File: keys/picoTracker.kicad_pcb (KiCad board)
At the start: 2 copper layers, 75 x 64.5 mm, 15 parts, among them J1 Conn_01x10, SW1 LEFT, SW2 DOWN, SW3 RIGHT, SW4 UP, SW5 LT, SW6 B, SW7 A, SW8 RT, SW9 PLAY

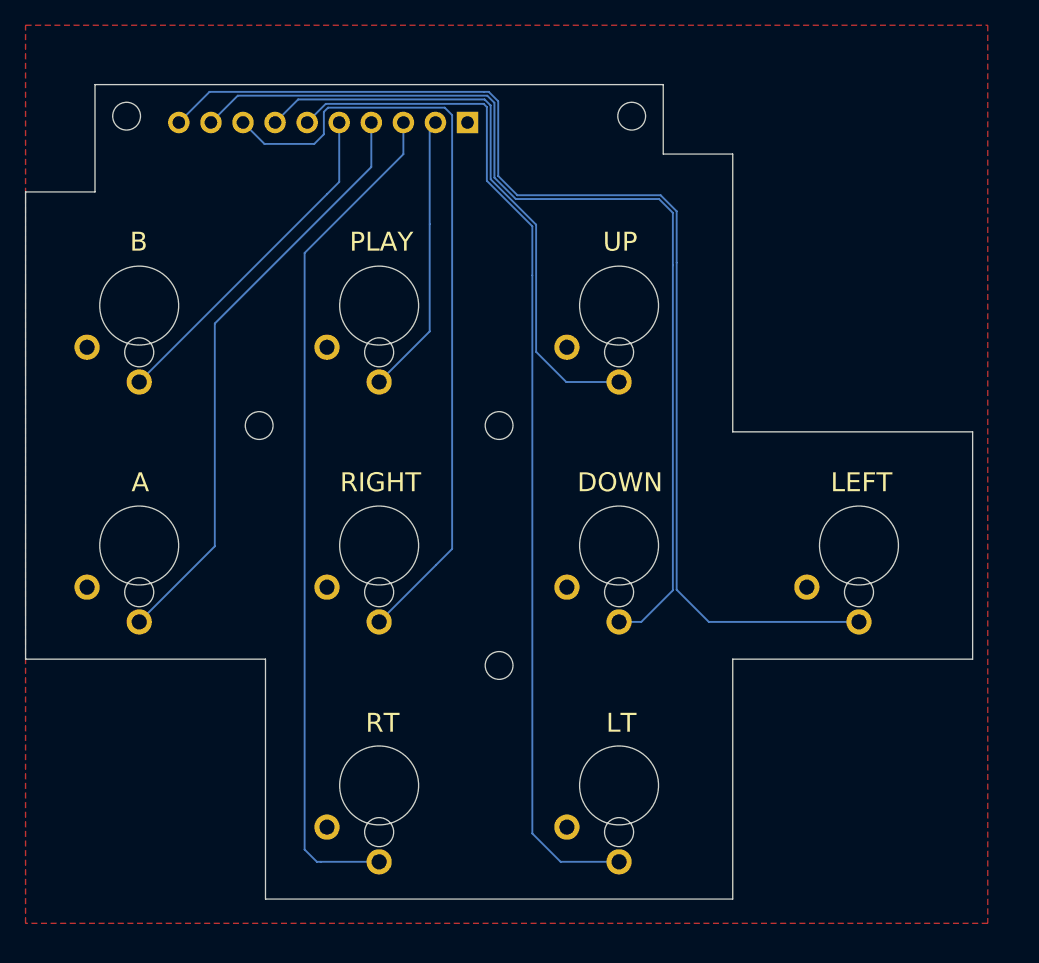
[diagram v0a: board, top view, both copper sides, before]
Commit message: picoTracker PCB v2.1 and picoTrackerKeypad PCB v2.0
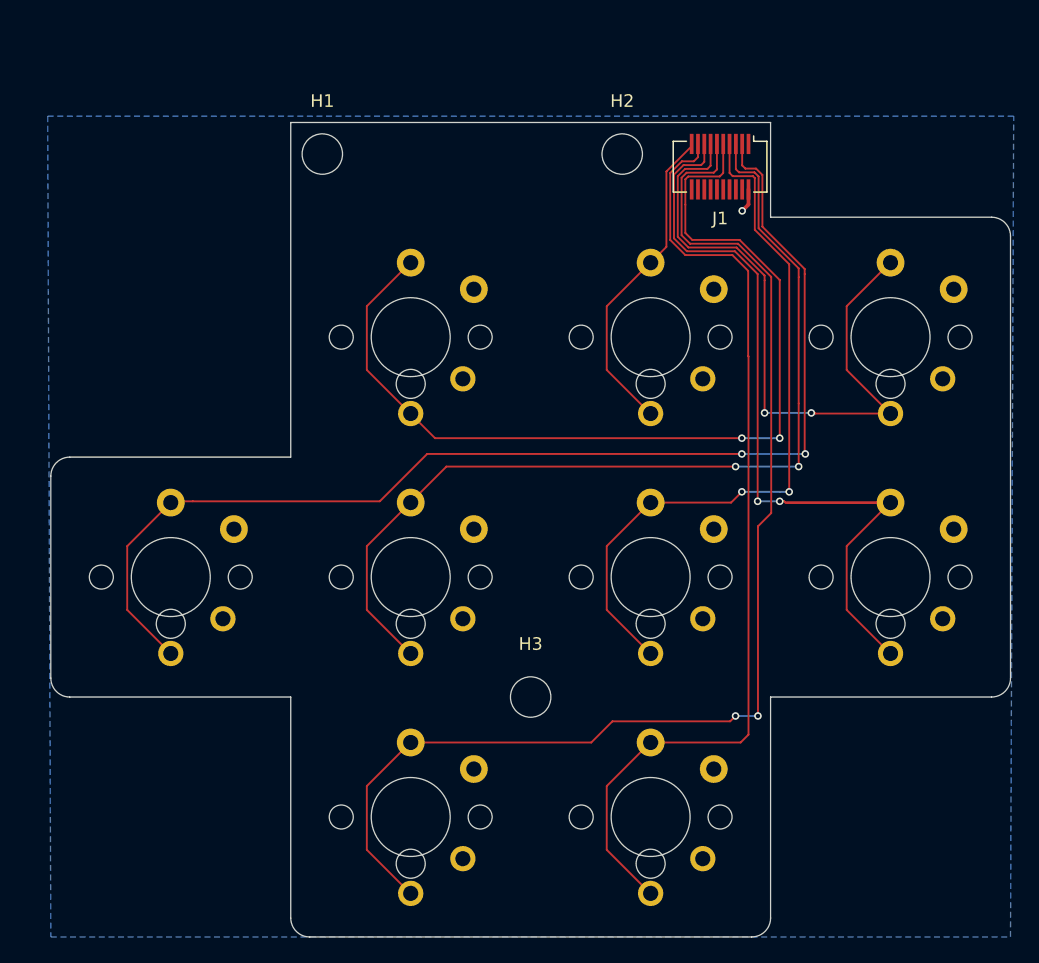
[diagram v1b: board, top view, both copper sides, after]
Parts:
- removed H4, H5: MountingHole, MountingHole:MountingHole_2.2mm_M2
- removed SW1: LEFT, Cherry MX LP:Cherry-MX-Low-Profile
- removed SW2: DOWN, Cherry MX LP:Cherry-MX-Low-Profile
- added REF**: OSHW-Logo2_9.8x8mm_SilkScreen, Symbol:OSHW-Logo2_9.8x8mm_SilkScreen, B.Cu at (41.2, 89.6)
- added SW10: NAV, project:Cherry-MX-Low-Profile-kailh, F.Cu at (49.5, 113.5)
- added SW11: PLAY, project:Cherry-MX-Low-Profile-kailh, F.Cu at (49.5, 75.5)
- H1, H2, H3: footprint MountingHole:MountingHole_2.2mm_M2 -> MountingHole:MountingHole_3.2mm_M3
- J1: value Conn_01x10 -> DF12NC(5.0)-20DP-0.5V(51); footprint Connector_PinHeader_2.54mm:PinHeader_1x10_P2.54mm_Vertical -> Connector_Hirose:Hirose_DF12_DF12E3.0-20DP-0.5V_2x10_P0.50mm_Vertical; moved to F.Cu
- SW3: value RIGHT -> LEFT; footprint Cherry MX LP:Cherry-MX-Low-Profile -> project:Cherry-MX-Low-Profile-kailh; moved to F.Cu
- SW4: value UP -> DOWN; footprint Cherry MX LP:Cherry-MX-Low-Profile -> project:Cherry-MX-Low-Profile-kailh; moved to F.Cu
- SW5: value LT -> RIGHT; footprint Cherry MX LP:Cherry-MX-Low-Profile -> project:Cherry-MX-Low-Profile-kailh; moved to F.Cu
- SW6: value B -> UP; footprint Cherry MX LP:Cherry-MX-Low-Profile -> project:Cherry-MX-Low-Profile-kailh; moved to F.Cu
- SW7: value A -> ALT; footprint Cherry MX LP:Cherry-MX-Low-Profile -> project:Cherry-MX-Low-Profile-kailh; moved to F.Cu
- SW8: value RT -> EDIT; footprint Cherry MX LP:Cherry-MX-Low-Profile -> project:Cherry-MX-Low-Profile-kailh; moved to F.Cu
- SW9: value PLAY -> ENTER; footprint Cherry MX LP:Cherry-MX-Low-Profile -> project:Cherry-MX-Low-Profile-kailh; moved to F.Cu
- moved SW8 53.9 mm to (68.5, 75.5), turned to 0 degrees
- moved SW9 45.9 mm to (68.5, 94.5), turned to 0 degrees
- moved H2 39.4 mm to (47.2, 61.0)
- moved SW7 30.4 mm to (30.5, 113.5), turned to 0 degrees
- moved SW4 27.1 mm to (30.5, 94.5), turned to 0 degrees
- moved H1 24.7 mm to (23.5, 61.0)
- moved H3 21.6 mm to (40.0, 104.0)
- moved SW6 21.6 mm to (30.5, 75.5), turned to 0 degrees
- moved J1 20.3 mm to (55.0, 62.0), turned to 180 degrees
- moved SW3 16.7 mm to (11.5, 94.5), turned to 0 degrees
- moved SW5 16.7 mm to (49.5, 94.5), turned to 0 degrees
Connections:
- net /SW_B renamed /INPUT_UP
- J1 pad 1: /GND -> +3.3V
- J1 pad 10: /SW_LEFT -> /INPUT_PLAY
- J1 pad 2: /SW_PLAY -> /INPUT_LEFT
- J1 pad 3: /SW_RT -> /INPUT_DOWN
- J1 pad 4: /SW_A -> /INPUT_RIGHT
- J1 pad 6: /SW_LT -> /INPUT_ALT
- J1 pad 7: /SW_UP -> /INPUT_EDIT
- J1 pad 8: /SW_RIGHT -> /INPUT_ENTER
- J1 pad 9: /SW_DOWN -> /INPUT_NAV
- SW3 pad 1: /SW_RIGHT -> /INPUT_LEFT
- SW3 pad 2: /GND -> GND
- SW4 pad 1: /SW_UP -> /INPUT_DOWN
- SW4 pad 2: /GND -> GND
- SW5 pad 1: /SW_LT -> /INPUT_RIGHT
- SW5 pad 2: /GND -> GND
- SW6 pad 2: /GND -> GND
- SW7 pad 1: /SW_A -> /INPUT_ALT
- SW7 pad 2: /GND -> GND
- SW8 pad 1: /SW_RT -> /INPUT_EDIT
- SW8 pad 2: /GND -> GND
- SW9 pad 1: /SW_PLAY -> /INPUT_ENTER
- SW9 pad 2: /GND -> GND
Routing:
- net /INPUT_ALT: track 0.00 -> 96.6 mm, vias 0 -> 2
- net /INPUT_LEFT: track 0.00 -> 93.8 mm, vias 0 -> 2
- net /SW_LEFT: track 93.3 -> 0.00 mm
- net /SW_LT: track 81.8 -> 0.00 mm
- net /SW_DOWN: track 80.0 -> 0.00 mm
- net /INPUT_NAV: track 0.00 -> 75.8 mm
- net /INPUT_DOWN: track 0.00 -> 75.1 mm, vias 0 -> 2
- net /INPUT_ENTER: track 0.00 -> 68.6 mm, vias 0 -> 2
- net /SW_RT: track 67.1 -> 0.00 mm
- net /SW_RIGHT: track 62.3 -> 0.00 mm
- net /INPUT_RIGHT: track 0.00 -> 56.6 mm, vias 0 -> 2
- net /INPUT_EDIT: track 0.00 -> 53.3 mm, vias 0 -> 2
- net /INPUT_UP: track 27.1 -> 76.2 mm, vias 0 -> 2
- net /SW_A: track 47.7 -> 0.00 mm
- net /SW_UP: track 46.6 -> 0.00 mm
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- added copper zone on B.Cu, net GND
- removed copper zone on F.Cu, net /GND
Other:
- board size 75 x 64.5 mm -> 76 x 64.5 mm
- board text added: "xiphonics PicoTrackerKeypad v2.0"
- board text removed: "A"
- board text removed: "B"
- board text removed: "DOWN"
- board text removed: "LEFT"
- board text removed: "LT"
- board text removed: "PLAY"
- board text removed: "RIGHT"
- board text removed: "RT"
- board text removed: "UP"
- board text removed: "https://github.com/democloid/picoTracker"
- board text removed: "picoTrackerPortable v1.0"
